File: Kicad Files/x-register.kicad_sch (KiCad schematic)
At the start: 20 parts, among them U43 74LS245, U44 74LS173, U45 74LS173

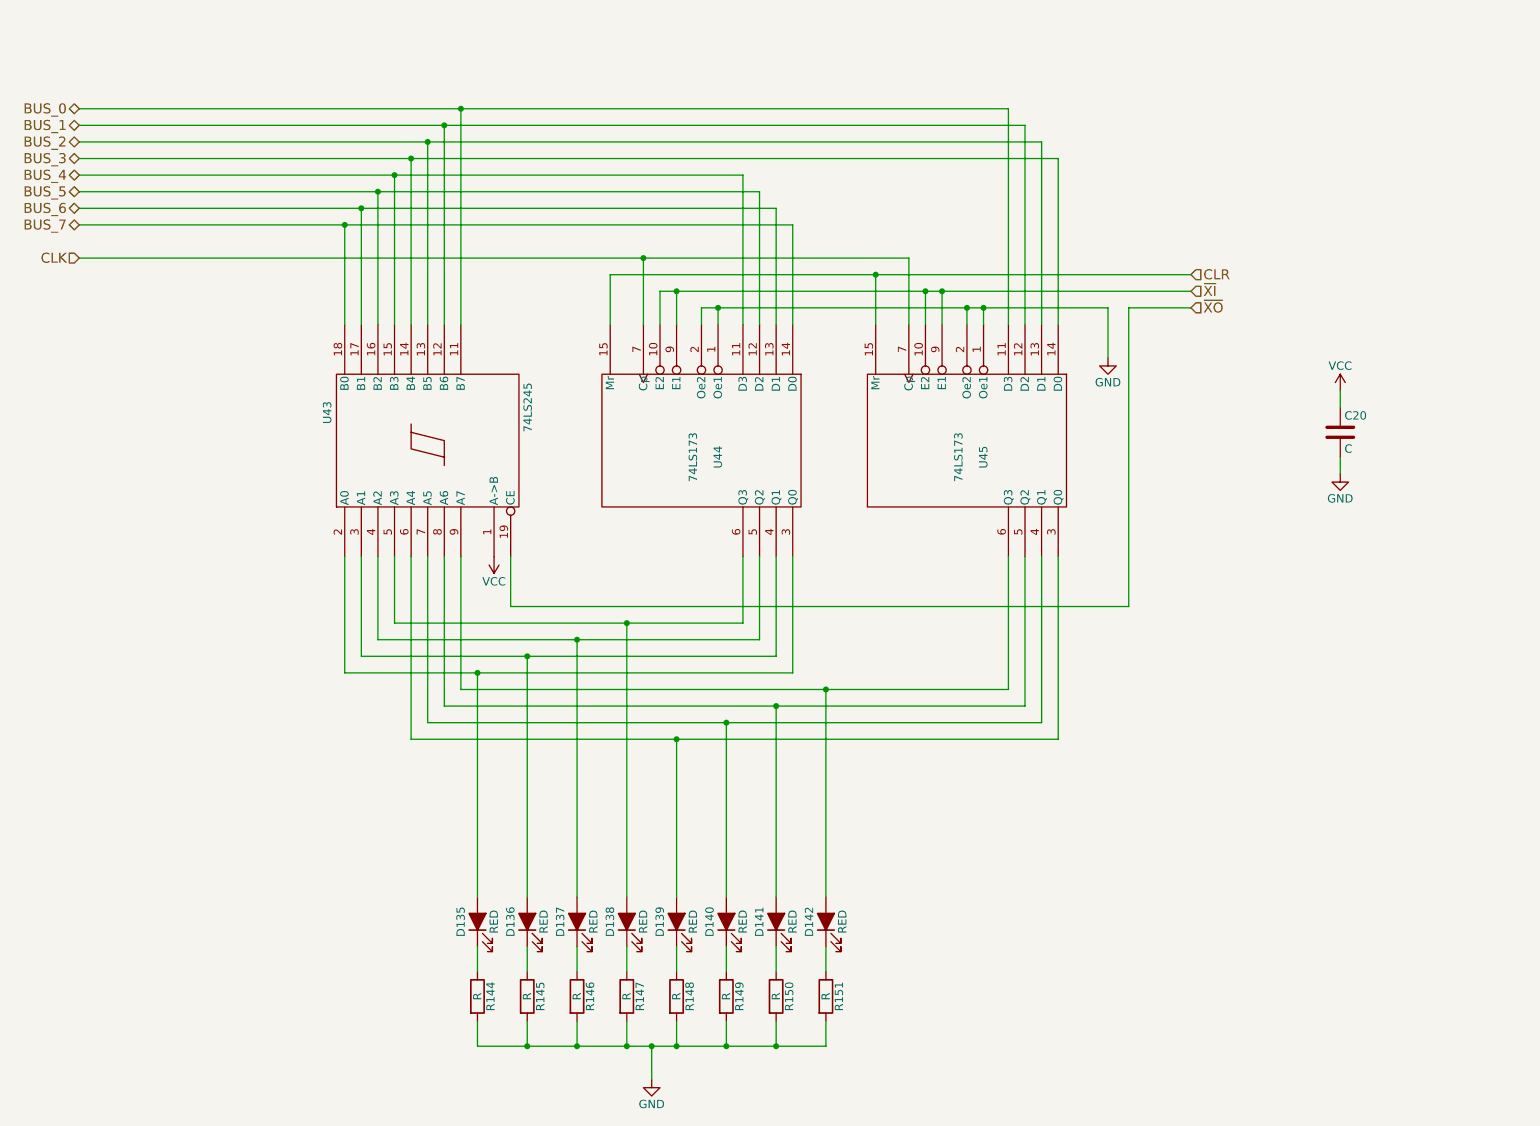
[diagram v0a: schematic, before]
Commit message: updated library
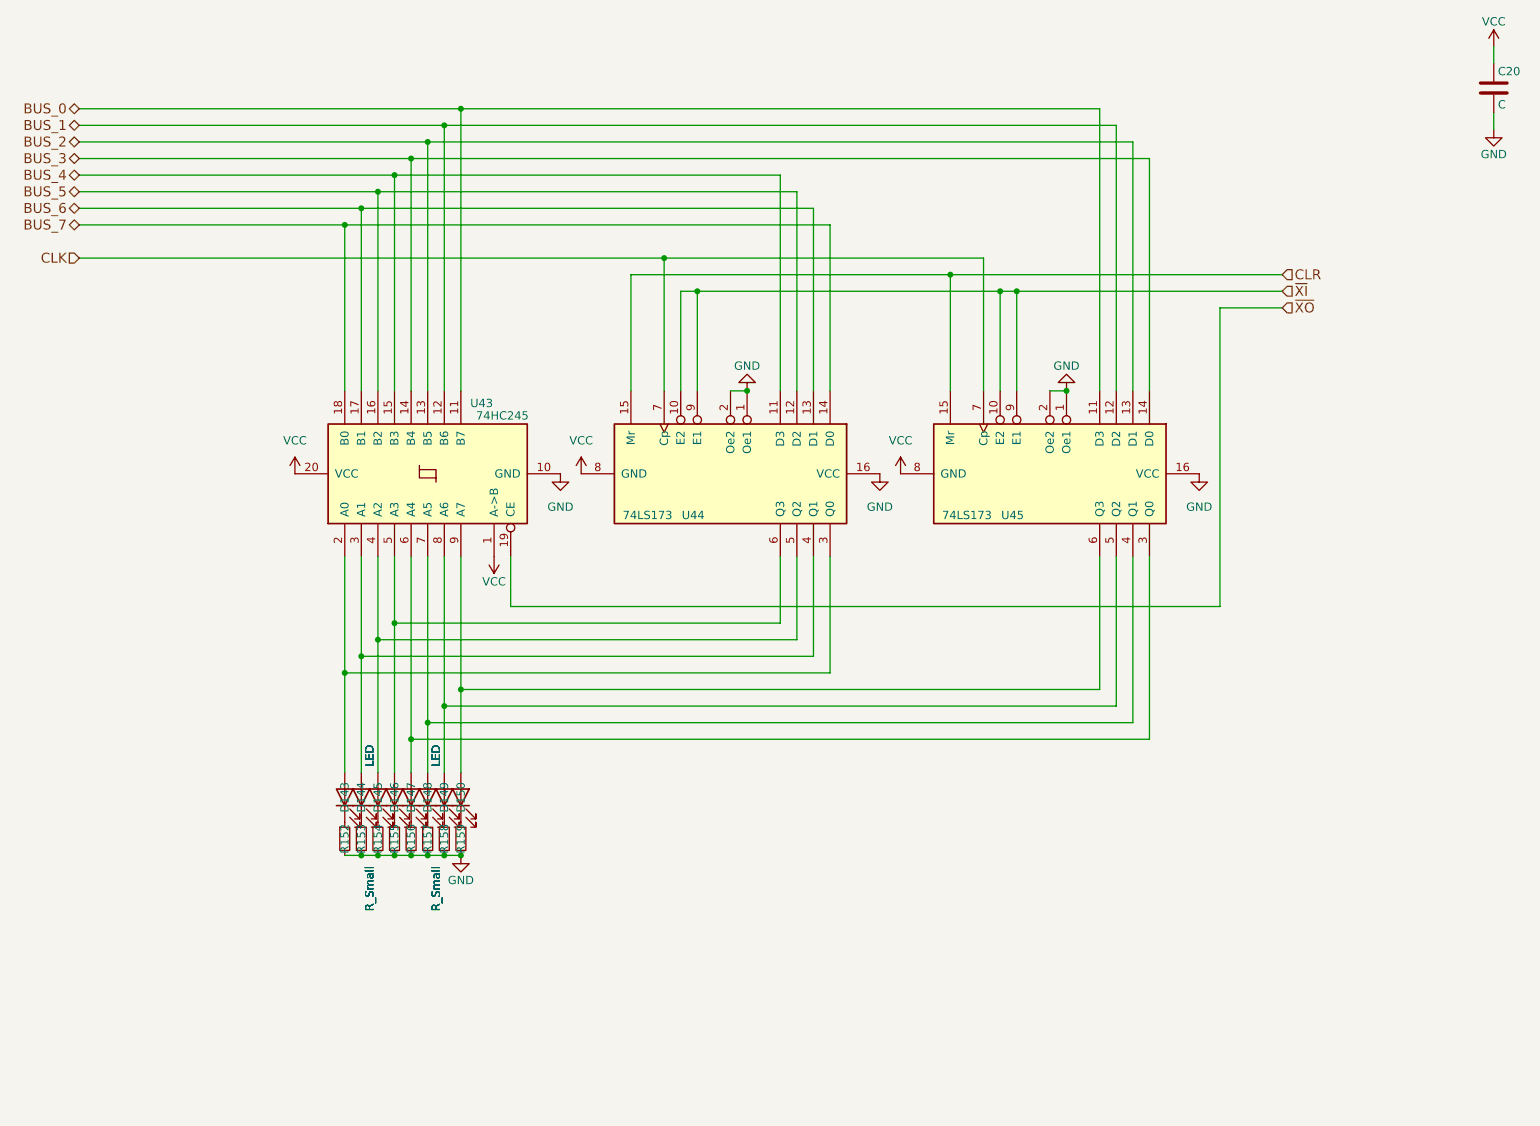
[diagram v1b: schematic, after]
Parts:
- removed D135, D136, D137, D138, D139, D140, D141, D142: RED, LED_THT:LED_D5.0mm, symbol 8bit-computer-rescue:LED_ALT-Device
- removed R144, R145, R146, R147, R148, R149, R150, R151: R, Resistor_THT:R_Axial_DIN0207_L6.3mm_D2.5mm_P7.62mm_Horizontal, symbol Device:R
- removed U43: 74LS245, Package_DIP:DIP-20_W7.62mm, symbol 8bit-computer-rescue:74LS245-8bit-computer-rescue
- removed U44, U45: 74LS173, Package_DIP:DIP-16_W7.62mm, symbol 8bit-computer-rescue:74LS173-8bit-computer-rescue
- added D143, D144, D145, D146, D147, D148, D149, D150: LED, symbol Device:LED
- added R152, R153, R154, R155, R156, R157, R158, R159: R_Small, symbol Device:R_Small
- added U43: 74HC245, symbol 74xx:74HC245
- added U44, U45: 74LS173, symbol 74xx:74LS173
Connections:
- net BUS_0: now also U43.11 (B7), U45.11 (D3)
- net BUS_1: now also U43.12 (B6), U45.12 (D2)
- net BUS_2: now also U43.13 (B5), U45.13 (D1)
- net BUS_3: now also U43.14 (B4), U45.14 (D0)
- net BUS_4: now also U43.15 (B3), U44.11 (D3)
- net BUS_5: now also U43.16 (B2), U44.12 (D2)
- net BUS_6: now also U43.17 (B1), U44.13 (D1)
- net BUS_7: now also U43.18 (B0), U44.14 (D0)
- net CLK: now also U44.7 (Cp), U45.7 (Cp)
- net CLR: now also U44.15 (Mr), U45.15 (Mr)
- net GND: now also R152.2, R153.2, R154.2, R155.2, R156.2, R157.2, R158.2, R159.2, U43.10 (GND), U44.1 (Oe1), U44.16 (VCC), U44.2 (Oe2), U45.1 (Oe1), U45.16 (VCC), U45.2 (Oe2)
- net VCC: now also U43.1 (A->B), U43.20 (VCC), U44.8 (GND), U45.8 (GND)
- net ~{XI}: now also U44.10 (E2), U44.9 (E1), U45.10 (E2), U45.9 (E1)
- net ~{XO}: now also U43.19 (CE)
- new net: D149.1 (K), R158.1
- new net: D147.1 (K), R156.1
- new net: D144.1 (K), R153.1
- new net: D144.2 (A), U43.3 (A1), U44.4 (Q1)
- new net: D147.2 (A), U43.6 (A4), U45.3 (Q0)
- new net: D148.2 (A), U43.7 (A5), U45.4 (Q1)
- new net: D149.2 (A), U43.8 (A6), U45.5 (Q2)
- new net: D150.2 (A), U43.9 (A7), U45.6 (Q3)
- new net: D150.1 (K), R159.1
- new net: D146.1 (K), R155.1
- new net: D146.2 (A), U43.5 (A3), U44.6 (Q3)
- new net: D143.1 (K), R152.1
- new net: D143.2 (A), U43.2 (A0), U44.3 (Q0)
- new net: D145.1 (K), R154.1
- new net: D145.2 (A), U43.4 (A2), U44.5 (Q2)
- new net: D148.1 (K), R157.1
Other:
- moved on the sheet: C20
